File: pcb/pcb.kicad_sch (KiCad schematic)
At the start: 39 parts, among them J1 USB_C_Receptacle_USB2.0, Q1 NMOS, Q2 NMOS, U1 BQ297xy, U2 BQ27441-G1, U5 TLV70028_SOT353

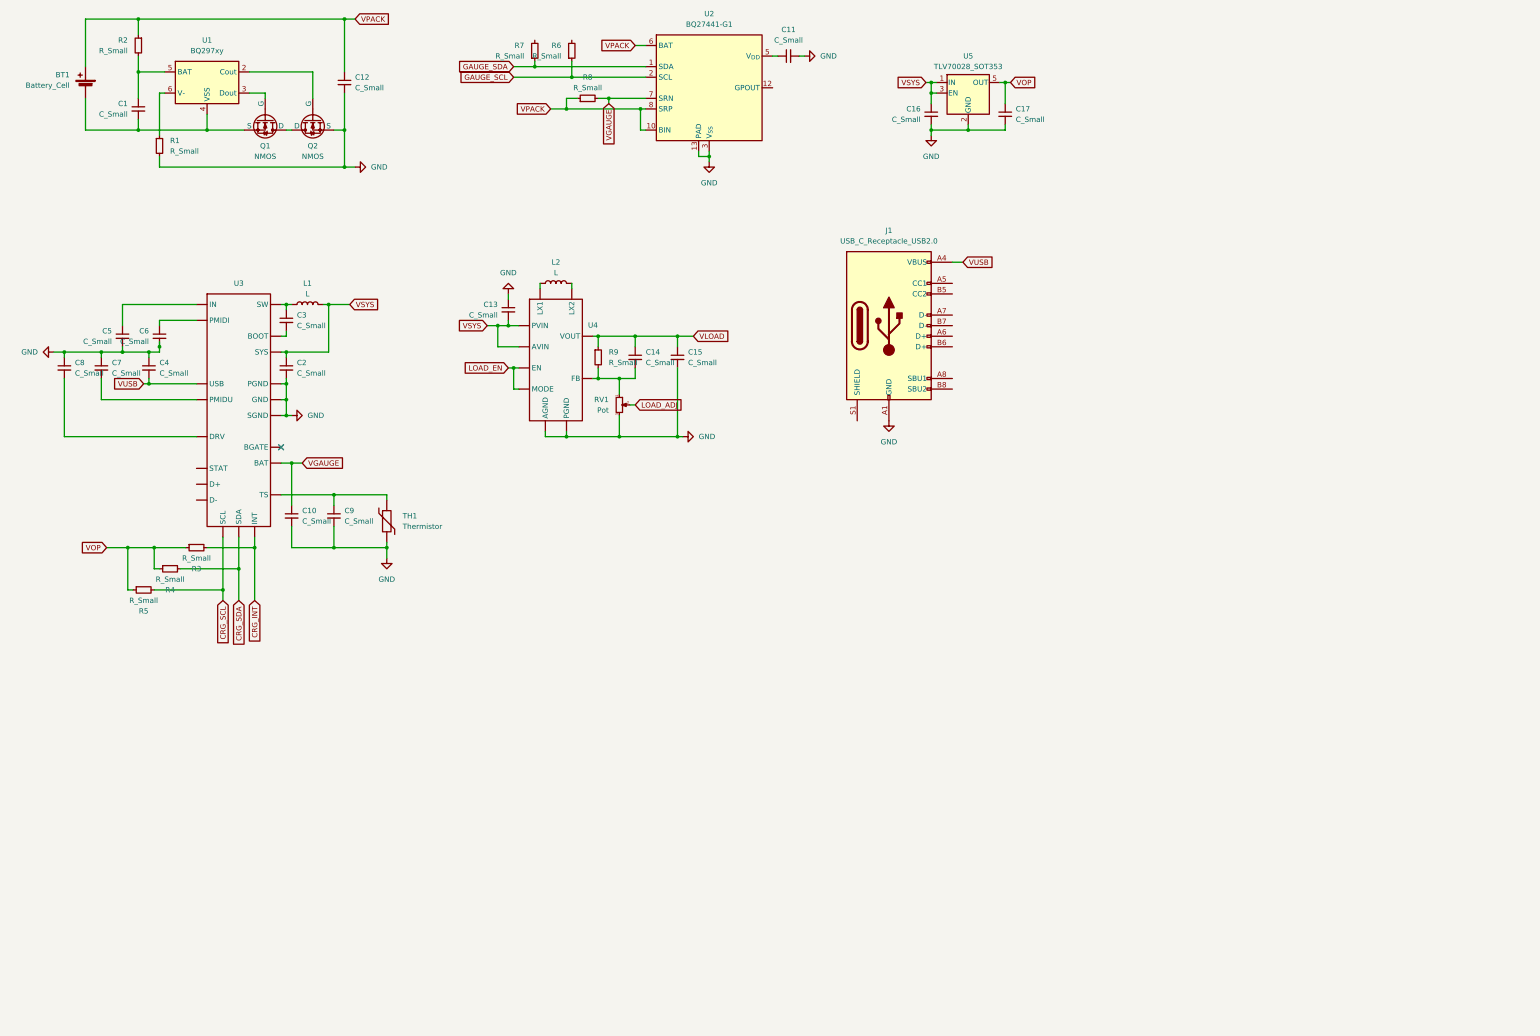
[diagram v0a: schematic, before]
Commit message: theres like... a cpu now
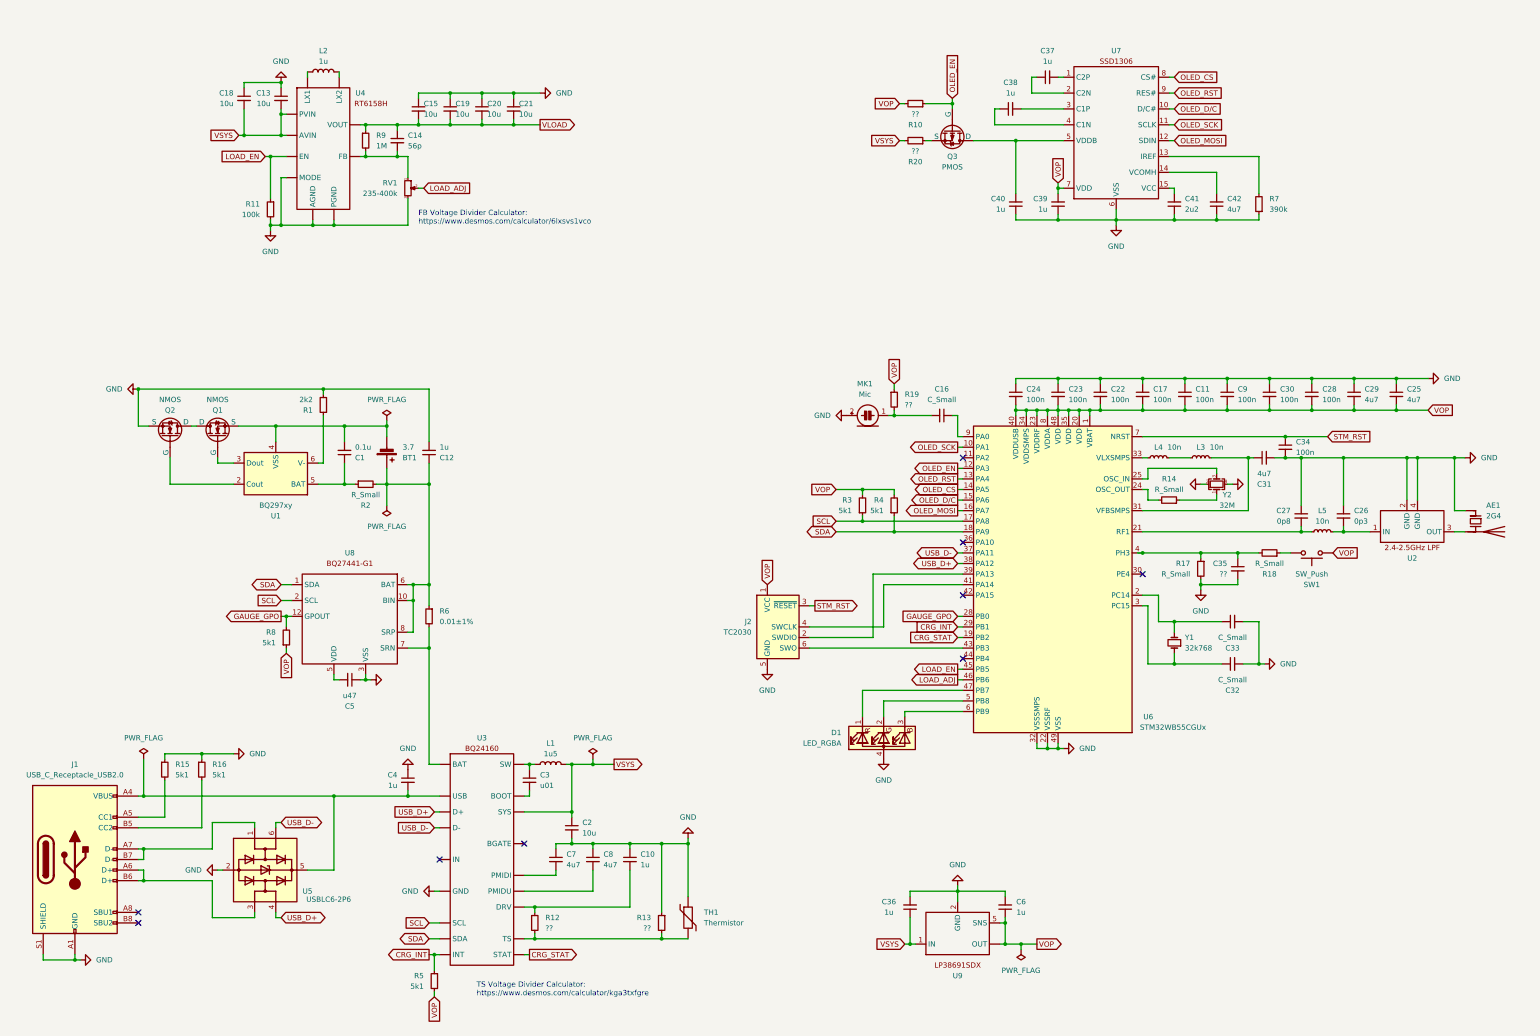
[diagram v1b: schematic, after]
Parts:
- removed U2: BQ27441-G1, Package_SON:Texas_S-PDSO-N12, symbol Battery_Management:BQ27441-G1
- removed U5: TLV70028_SOT353, Package_TO_SOT_SMD:SOT-353_SC-70-5, symbol Regulator_Linear:TLV70028_SOT353
- added AE1: 2G4, symbol Device:Antenna_Chip
- added C18, C19, C20, C21: 10u, symbol Device:C_Small
- added C22, C23, C24, C28, C30, C34: 100n, symbol Device:C_Small
- added C25, C29, C31, C42: 4u7, symbol Device:C_Small
- added C26: 0p3, symbol Device:C_Small
- added C27: 0p8, symbol Device:C_Small
- added C32, C33: C_Small, symbol Device:C_Small
- added C35: ??, symbol Device:C_Small
- added C36, C37, C38, C39, C40: 1u, symbol Device:C_Small
- added C41: 2u2, symbol Device:C_Small
- added D1: LED_RGBA, symbol Device:LED_RGBA
- added J2: TC2030, Connector:Tag-Connect_TC2030-IDC-FP_2x03_P1.27mm_Vertical, symbol Connector:Conn_ARM_SWD_TagConnect_TC2030
- added L3, L4, L5: 10n, symbol Device:L_Small
- added MK1: Mic, symbol Device:Microphone_Condenser
- added Q3: PMOS, symbol Simulation_SPICE:PMOS
- added R10, R12, R13, R19, R20: ??, symbol Device:R_Small
- added R11: 100k, symbol Device:R_Small
- added R14, R17, R18: R_Small, symbol Device:R_Small
- added R15, R16: 5k1, symbol Device:R_Small
- added SW1: SW_Push, symbol Switch:SW_Push
- added U2: ~, symbol symbol_library:DLF162500LT-5028A1
- added U5: USBLC6-2P6, Package_TO_SOT_SMD:SOT-666, symbol Power_Protection:USBLC6-2P6
- added U6: STM32WB55CGUx, Package_DFN_QFN:QFN-48-1EP_7x7mm_P0.5mm_EP5.6x5.6mm, symbol MCU_ST_STM32WB:STM32WB55CGUx
- added U7: ~, symbol symbol_library:SSD1306
- added U8: ~, symbol symbol_library:BQ27441-G1
- added U9: ~, symbol symbol_library:LP38691SDX-3.3/NOPB
- added Y1: 32k768, symbol Device:Crystal_Small
- added Y2: 32M, symbol Device:Crystal_GND24_Small
- BT1: value Battery_Cell -> 3.7
- C1: value C_Small -> 0.1u
- C10, C12, C4, C6: value C_Small -> 1u
- C11, C17, C9: value C_Small -> 100n
- C13, C15, C2: value C_Small -> 10u
- C14: value C_Small -> 56p
- C3: value C_Small -> u01
- C5: value C_Small -> u47
- C7, C8: value C_Small -> 4u7
- L1: value L -> 1u5
- L2: value L -> 1u
- R1: value R_Small -> 2k2
- R3, R4, R5, R8: value R_Small -> 5k1
- R6: value R_Small -> 0.01±1%
- R7: value R_Small -> 390k
- R9: value R_Small -> 1M
- RV1: value Pot -> 235-400k
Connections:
- net GAUGE_SDA is gone; now on net GND: R7.1
- net CRG_INT: now also R5.1, U6.29 (PB1); no longer R3.2
- net GND: now also C10.1, C11.1, C15.1, C17.1, C5.1, C9.1, J1.S1 (SHIELD), TH1.1, AE1.1 (FEED), C18.1, C19.1, C20.1, C21.1, C22.1, C23.1, C24.1, C25.1, C26.1, C27.1, C28.1, C29.1, C30.1, C31.2, C32.2, C33.2, C34.2, C35.2, C36.2, C39.1, C40.1, C41.1, C42.1, D1.4 (A), J2.5 (GND), MK1.2 (+), R11.2, R13.1, R15.1, R16.1, R17.2, U2.2 (GND), U2.4 (GND), U5.2 (GND), U6.22 (VSSRF), U6.32 (VSSSMPS), U6.49 (VSS), U7.6 (VSS), U8.3 (VSS), U9.2 (GND), Y2.2, Y2.4; no longer C10.2, C11.2, C15.2, C16.2, C17.2, C5.2, C9.2, TH1.2
- net LOAD_ADJ: now also U6.46 (PB6)
- net LOAD_EN: now also R11.1, U6.45 (PB5)
- net VLOAD: now also C15.2, C19.2, C20.2, C21.2; no longer C15.1
- net VOP: now also C11.2, C17.2, C6.1, C9.2, R3.2, R4.2, R5.2, R8.1, C22.2, C23.2, C24.2, C25.2, C28.2, C29.2, C30.2, C39.2, J2.1 (VCC), R10.2, R19.1, SW1.1, U6.1 (VBAT), U6.20 (VDD), U6.23 (VDDRF), U6.34 (VDDSMPS), U6.35 (VDD), U6.40 (VDDUSB), U6.48 (VDD), U6.8 (VDDA), U7.7 (VDD), U9. (OUT), U9.5 (SNS); no longer C17.1, R3.1, R4.1, R5.1
- net VSYS: now also C18.2, C36.1, R20.2, U9.1 (IN); no longer C16.1
- net at C1.1, U1.5 (BAT): now also R2.1; no longer R2.2
- net at R6.2: now also U3. (USB), U8.7 (SRN)
- net at R7.2: now also U7.13 (IREF)
- net at J1.A5 (CC1): now also R15.2
- net at J1.A6 (D+): now also J1.B6 (D+), U5.3 (I/O2)
- net at J1.A7 (D-): now also J1.B7 (D-), U5.1 (I/O1)
- net at J1.B5 (CC2): now also R16.2
- removed net CRG_SCL: R5.2, U3. (USB)
- removed net CRG_SDA: R4.2, U3. (USB)
- net GAUGE_SCL: no longer names the net of R6.1
- net GAUGE_SCL: now also BT1.1 (+), C12.1, R2.2, U8.10 (BIN), U8.6 (BAT), U8.8 (SRP)
- removed net VGAUGE: C10.1, R8.2, U3. (USB)
- removed net VPACK: BT1.1 (+), C12.1, R2.1, R8.1
- net VUSB: no longer names the net of C4.2, J1.A4 (VBUS), J1.A9 (VBUS), J1.B4 (VBUS), J1.B9 (VBUS), U3. (USB)
- net VUSB: now also U5.5 (VBUS)
- new net: C26.2, L5.1, U2.1 (IN)
- new net: R14.1, Y2.1
- new net: R14.2, U6.24 (OSC_OUT)
- new net: C27.2, L5.2, U6.21 (RF1)
- new net: C33.1, U6.2 (PC14), Y1.2
- new net: U6.25 (OSC_IN), Y2.3
- new net: C32.1, U6.3 (PC15), Y1.1
- new net: C31.1, L3.1, U6.31 (VFBSMPS)
- new net: L4.2, U6.33 (VLXSMPS)
- new net: J2.2 (SWDIO), U6.39 (PA13)
- new net: C35.1, R17.1, R18.2, U6.4 (PH3)
- new net: J2.4 (SWCLK), U6.41 (PA14)
- new net: J2.6 (SWO), U6.43 (PB3)
- new net: D1.1 (RK), U6.47 (PB7)
- new net: D1.2 (GK), U6.5 (PB8)
- new net: D1.3 (BK), U6.6 (PB9)
- new net: C16.1, U6.9 (PA0)
- new net: L3.2, L4.1
- new net: C41.2, U7.15 (VCC)
- new net: C37.2, U7.1 (C2P)
- new net: C42.2, U7.14 (VCOMH)
- new net: C37.1, U7.2 (C2N)
- new net: C38.2, U7.3 (C1P)
- new net: C38.1, U7.4 (C1N)
- new net: C40.2, Q3.1 (D), U7.5 (VDDB)
- new net: C10.2, R12.1, U3. (USB)
- new net: R12.2, R13.2, TH1.2, U3. (USB)
- new net: C16.2, MK1.1 (-), R19.2
- new net: C5.2, U8.5 (VDD)
- new net: AE1.2 (PCB_Trace), U2.3 (OUT)
- new net: R18.1, SW1.2
- new net: Q3.3 (S), R20.1
- new net CRG_STAT: U3. (USB), U6.19 (PB2)
- new net GAUGE_GPO: R8.2, U6.28 (PB0), U8.12 (GPOUT)
- new net OLED_CS: U6.14 (PA5), U7.8 (CS#)
- new net OLED_D/C: U6.15 (PA6), U7.10 (D/C#)
- new net OLED_EN: Q3.2 (G), R10.1, U6.12 (PA3)
- new net OLED_MOSI: U6.16 (PA7), U7.12 (SDIN)
- new net OLED_RST: U6.13 (PA4), U7.9 (RES#)
- new net OLED_SCK: U6.10 (PA1), U7.11 (SCLK)
- new net SCL: R3.1, U3. (USB), U6.17 (PA8), U8.2 (SCL)
- new net SDA: R4.1, U3. (USB), U6.18 (PA9), U8.1 (SDA)
- new net STM_RST : C34.1, J2.3 (~{RESET}), U6.7 (NRST)
- new net USB_D+: U3. (USB), U5.4 (I/O2), U6.38 (PA12)
- new net USB_D-: U3. (USB), U5.6 (I/O1), U6.37 (PA11)
- no-connect marks 1 -> 9
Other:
- note added: "FB Voltage Divider Calculator: https://www.desmos.com/calculator/6lxsvs1vco"
- note added: "TS Voltage Divider Calculator: https://www.desmos.com/calculator/kga3txfgre"
- moved on the sheet: BT1, C1, C10, C12, C13, C14, C15, C3, C7, C8, J1, L1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

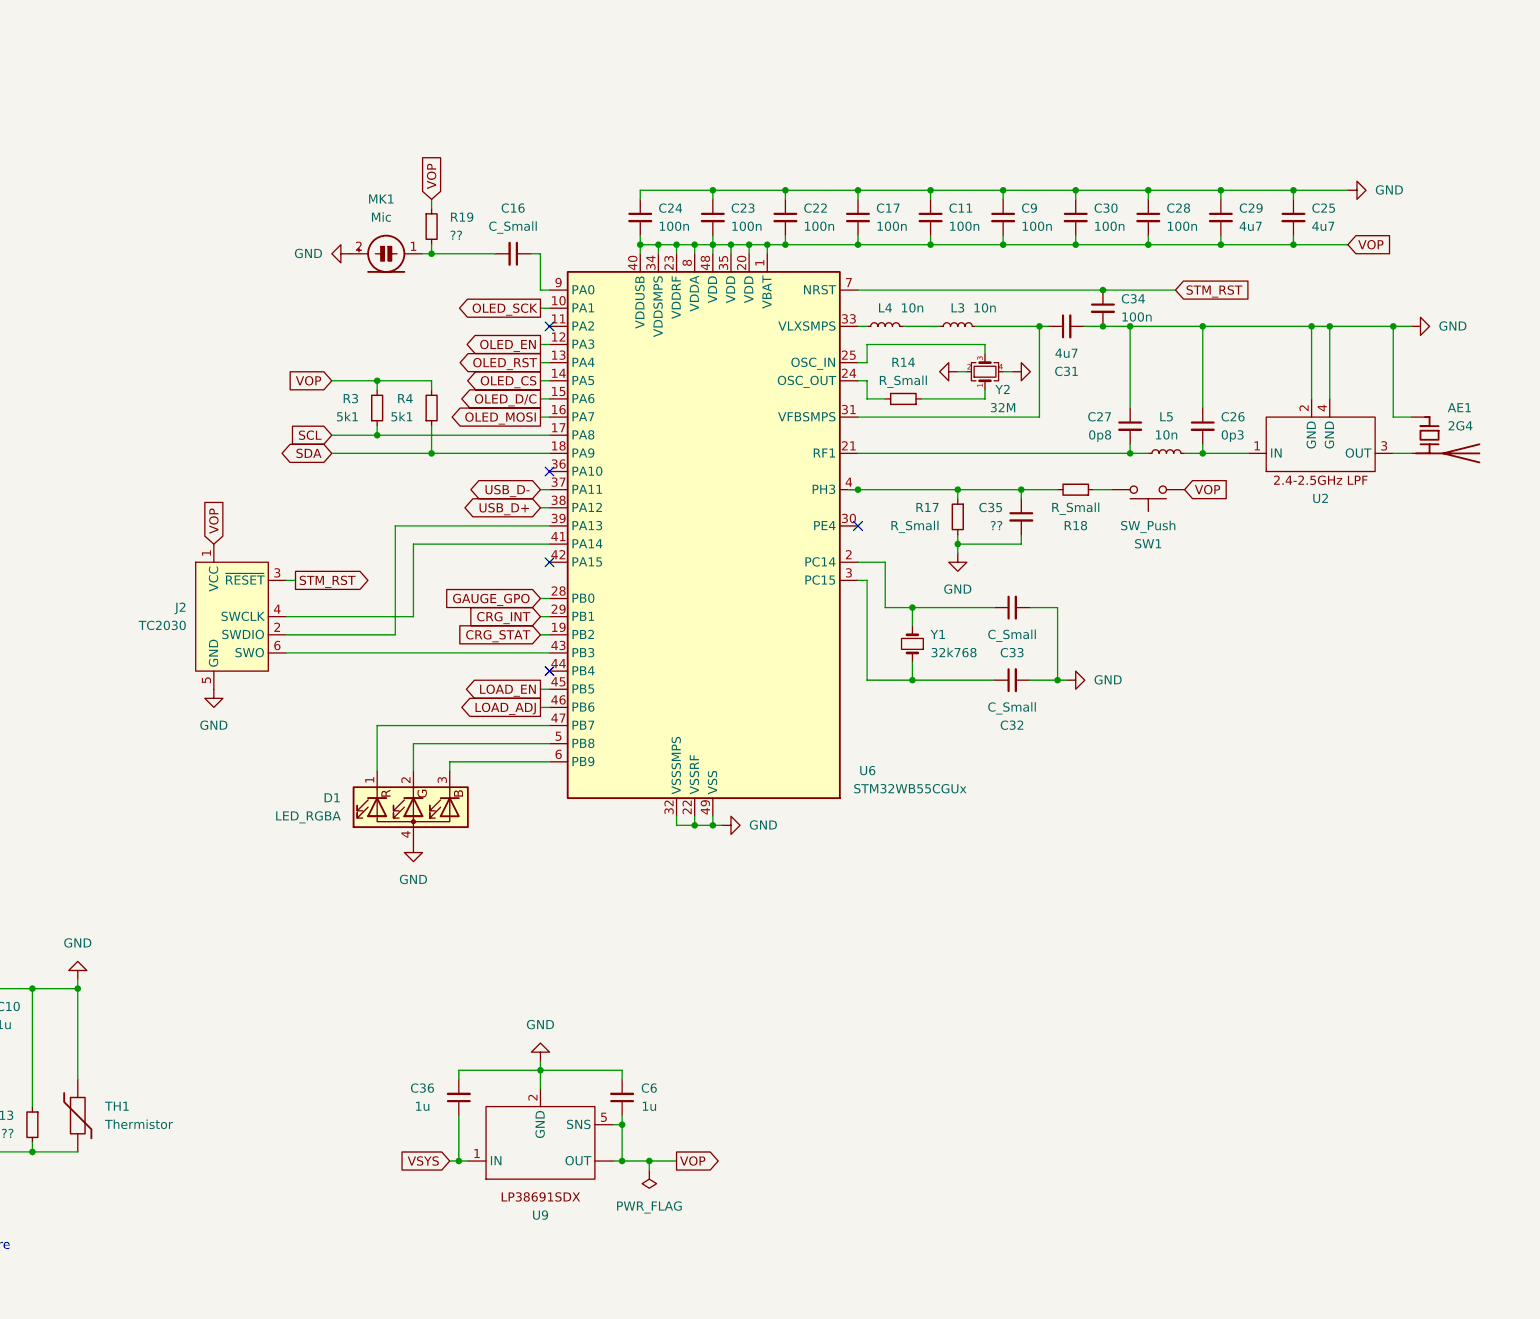
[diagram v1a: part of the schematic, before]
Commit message: schematic stuff
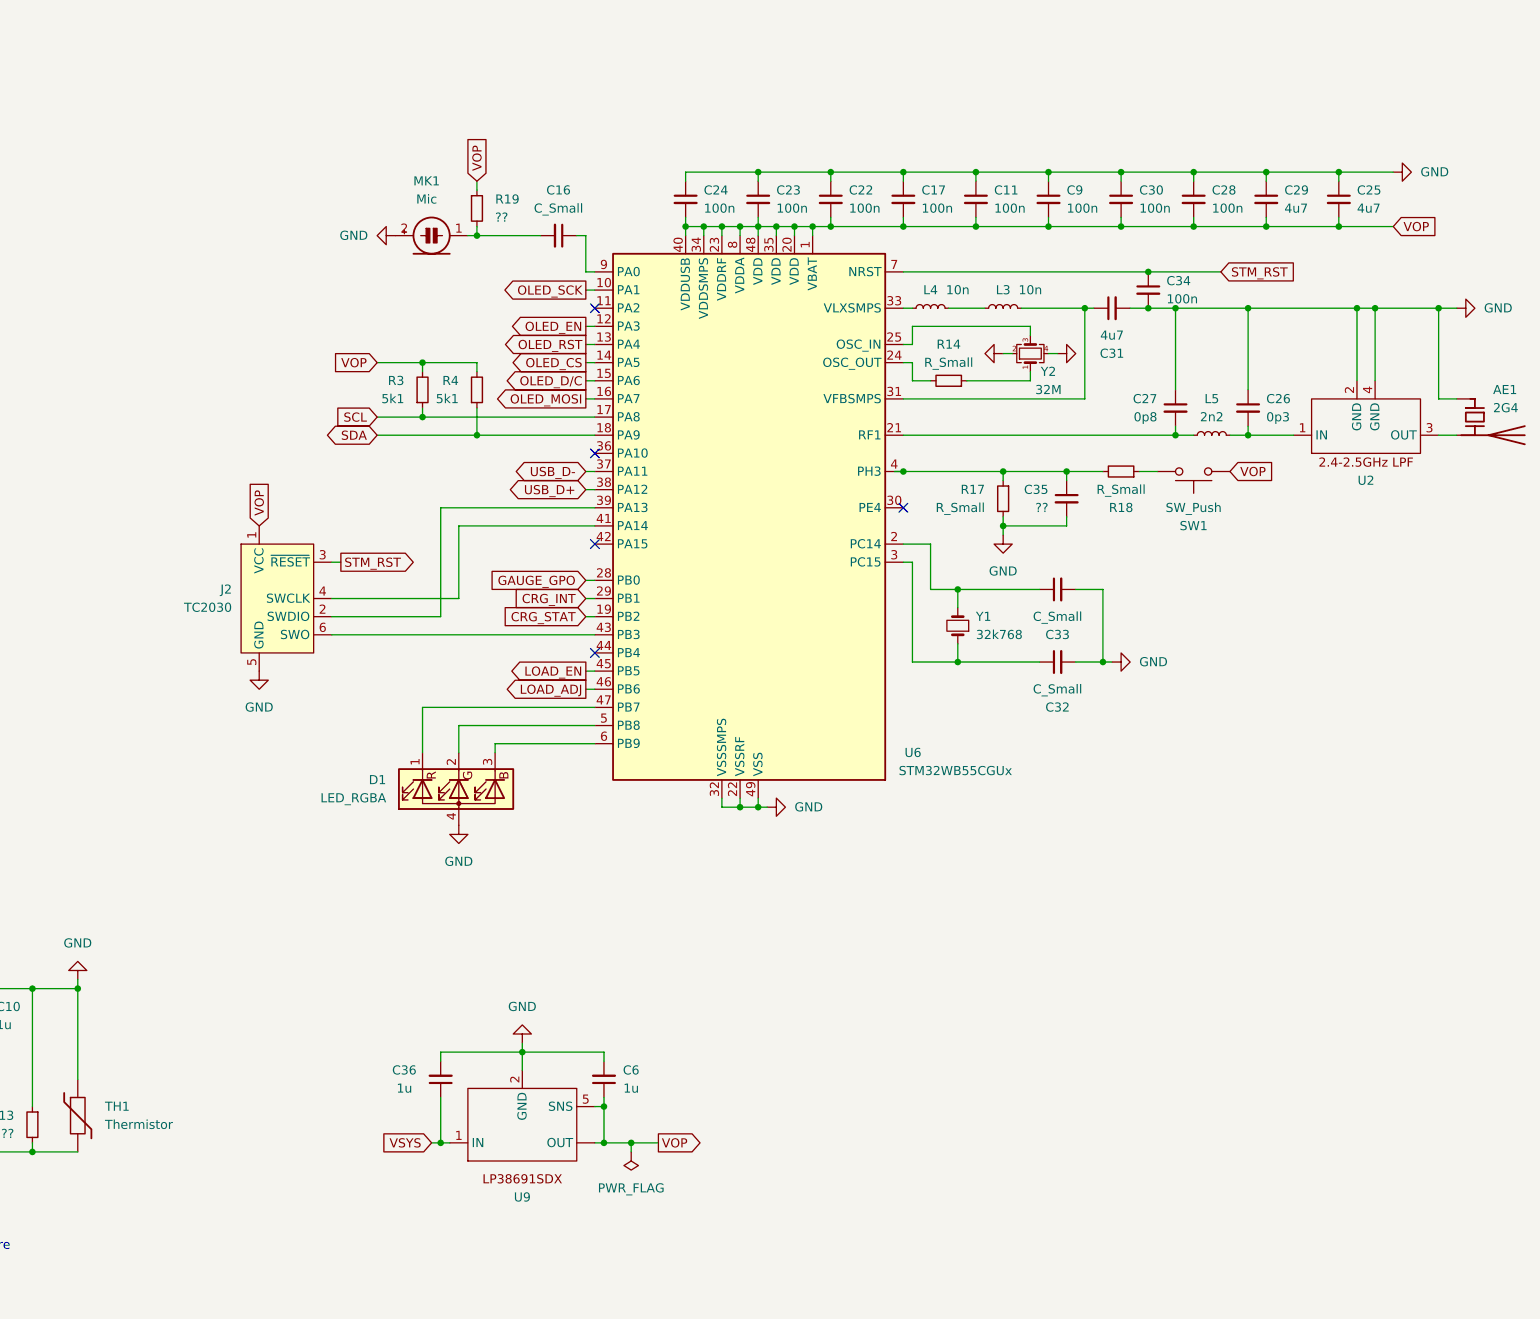
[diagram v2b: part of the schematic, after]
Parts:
- AE1: Distrubuter Link (none) -> https://www.digikey.com/en/products/detail/johanson-technol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
- BT1: Distrubuter Link (none) -> https://www.digikey.com/en/products/detail/jauch-quartz/LI1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
- D1: Distrubuter Link (none) -> https://www.digikey.com/en/products/detail/rohm-semiconduct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
- L5: value 10n -> 2n2
- Q1, Q2, U1, U3, U8, U9: Distrubuter Link (none) -> https://www.digikey.com/en/products/detail/texas-instrument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
- R6: footprint (none) -> Resistor_SMD:R_1206_3216Metric; Distrubuter Link (none) -> https://www.digikey.com/en/products/detail/ohmite/MCS1632R0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
- U2: Distrubuter Link (none) -> https://www.digikey.com/en/products/detail/tdk-corporation/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
- U4: Distrubuter Link (none) -> https://www.digikey.com/en/products/detail/richtek-usa-inc/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
- U5, U6: Distrubuter Link (none) -> https://www.digikey.com/en/products/detail/stmicroelectroni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
- U7: Distrubuter Link (none) -> https://www.digikey.com/en/products/detail/midas-displays/M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
- Y1: Distrubuter Link (none) -> https://www.digikey.com/en/products/detail/ndk-america-inc/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
- Y2: Distrubuter Link (none) -> https://www.digikey.com/en/products/detail/ecliptek/EC3625E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
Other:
- moved on the sheet: AE1, C11, C16, C17, C22, C23, C24, C25, C26, C27, C28, C29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
